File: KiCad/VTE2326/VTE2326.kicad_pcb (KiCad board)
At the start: 2 copper layers, 77.5 x 50 mm, 24 parts, among them J1 Power, J3 Programer, M1 Motor_DC, SW1 Reset, SW2 Mode, U1 AMS1117-3.3, U2 ESP-12E, U3 NPK, U4 L293D, U5 AMS1117-5.0

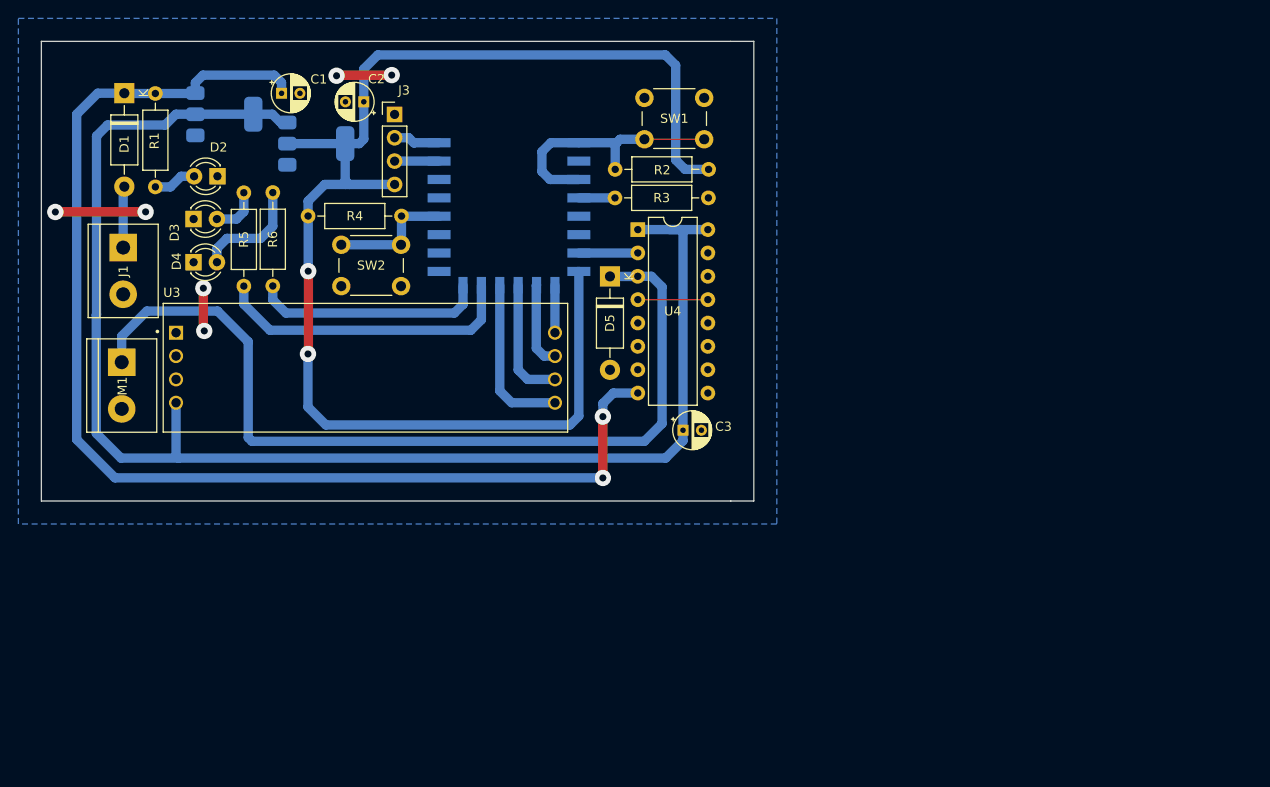
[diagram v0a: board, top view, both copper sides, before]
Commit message: Updates
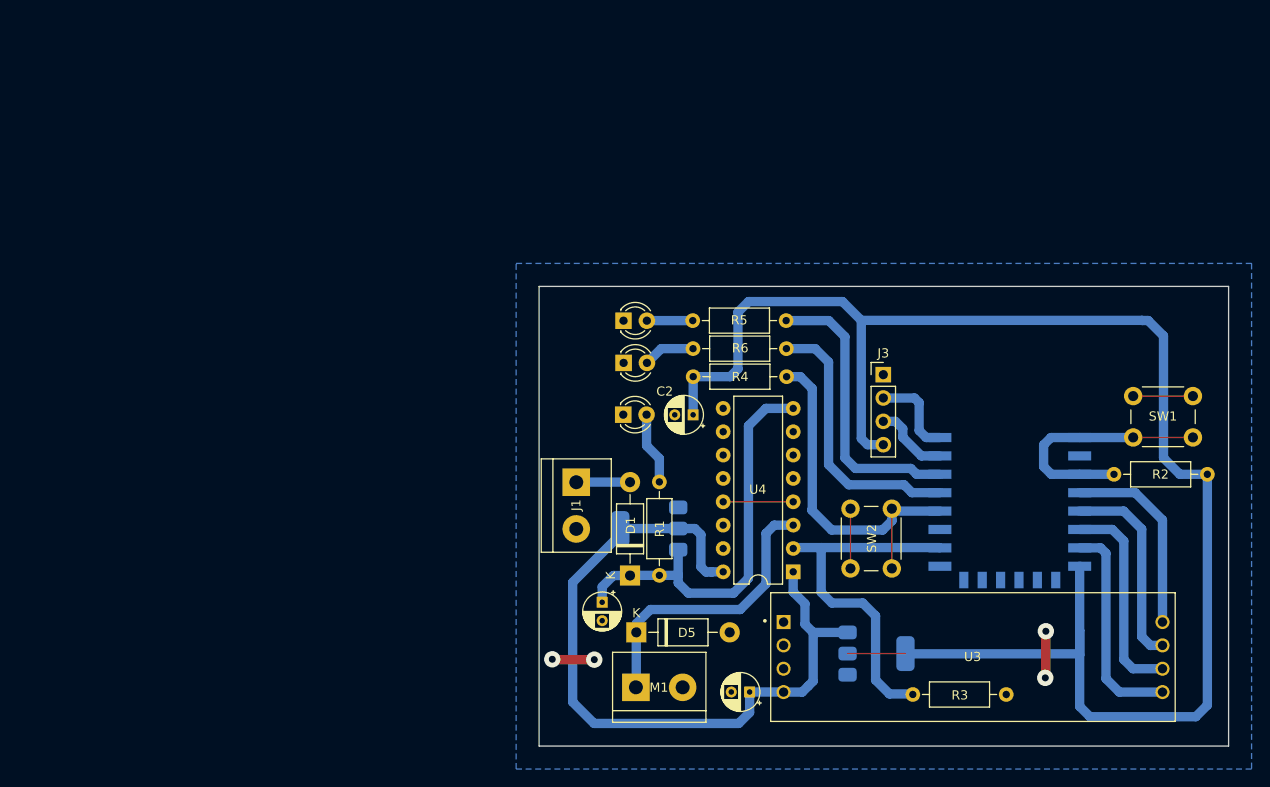
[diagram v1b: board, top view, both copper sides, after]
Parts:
- moved U1 82.4 mm to (209.2, 124.9)
- moved D1 76.0 mm to (182.4, 116.5), turned to 90 degrees
- moved R1 75.8 mm to (185.6, 116.4), turned to 90 degrees
- moved U3 73.2 mm to (219.7, 125.3)
- moved SW2 66.4 mm to (210.9, 109.2), turned to -90 degrees
- moved M1 66.2 mm to (183.0, 128.6), turned to 0 degrees
- moved C1 65.4 mm to (179.4, 119.4), turned to -90 degrees
- moved U5 64.6 mm to (184.5, 111.3), turned to 180 degrees
- moved R2 63.6 mm to (245.2, 105.4)
- moved U2 63.2 mm to (223.7, 104.9)
- moved R3 63.0 mm to (213.2, 129.4)
- moved SW1 62.3 mm to (237.1, 96.9)
- moved J3 60.2 mm to (209.9, 94.6)
- moved R5 59.1 mm to (199.4, 88.7), turned to 180 degrees
- moved J1 55.5 mm to (176.5, 106.3)
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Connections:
- R3 pad 1: Net-(U2-GPIO16) -> /pump
- R5 pad 1: Net-(U2-MOSI) -> Net-(U2-GPIO5)
- R6 pad 2: Net-(U2-SCLK) -> Net-(U2-GPIO4)
- U2 pad 10: /DE -> unconnected-(U2-MISO-Pad10)
- U2 pad 11: /RE -> unconnected-(U2-GPIO9-Pad11)
- U2 pad 12: /RO -> unconnected-(U2-GPIO10-Pad12)
- U2 pad 13: Net-(U2-MOSI) -> unconnected-(U2-MOSI-Pad13)
- U2 pad 14: Net-(U2-SCLK) -> unconnected-(U2-SCLK-Pad14)
- U2 pad 16: unconnected-(U2-GPIO15-Pad16) -> /pump
- U2 pad 19: unconnected-(U2-GPIO4-Pad19) -> Net-(U2-GPIO4)
- U2 pad 20: unconnected-(U2-GPIO5-Pad20) -> Net-(U2-GPIO5)
- U2 pad 4: Net-(U2-GPIO16) -> /DI
- U2 pad 5: unconnected-(U2-GPIO14-Pad5) -> /DE
- U2 pad 6: unconnected-(U2-GPIO12-Pad6) -> /RE
- U2 pad 7: /pump -> /RO
- U2 pad 9: /DI -> unconnected-(U2-CS0-Pad9)
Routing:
- net +12V: track 133.0 -> 45.1 mm, vias 2 -> 0
- net +5V: track 158.3 -> 83.1 mm
- net Net-(D5-K): track 96.5 -> 31.7 mm
- net Net-(U2-MOSI): track 33.2 -> 0.00 mm
- net /pump: track 6.42 -> 39.5 mm
- net +3.3V: track 149.1 -> 181.4 mm
- net Net-(U2-GPIO5): track 0.00 -> 31.4 mm
- net Net-(U2-GPIO4): track 0.00 -> 29.7 mm
- net Net-(SW2A-A): track 13.7 -> 39.9 mm
- net Net-(U2-SCLK): track 25.3 -> 0.00 mm
- net /DI: track 5.17 -> 21.3 mm
- net /DE: track 9.26 -> 21.9 mm
- net /RE: track 13.6 -> 22.8 mm
- net Net-(D4-A): track 12.2 -> 5.65 mm
- net /RO: track 18.0 -> 23.5 mm
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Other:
- board size 77.5 x 50 mm -> 75 x 50 mm
